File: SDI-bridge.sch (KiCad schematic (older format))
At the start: 95 parts, among them J1 543630489, J2 031-70526-21, J3 3220-10-0100-00, U1 GS2971A, U2 MAX8902B, Y1 ABM7_27.000MH_D2Y_T

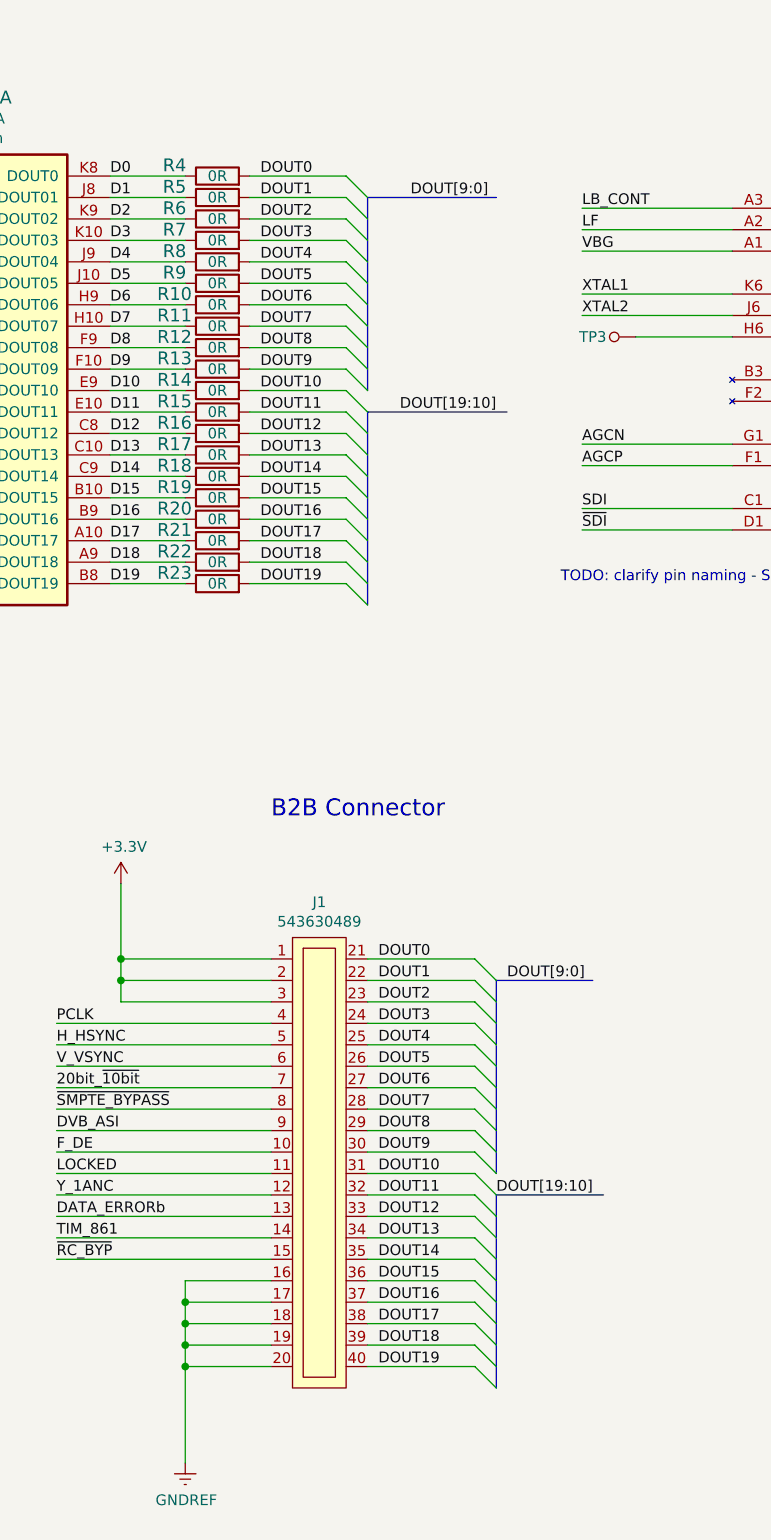
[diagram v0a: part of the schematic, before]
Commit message: Initial routing -WIP
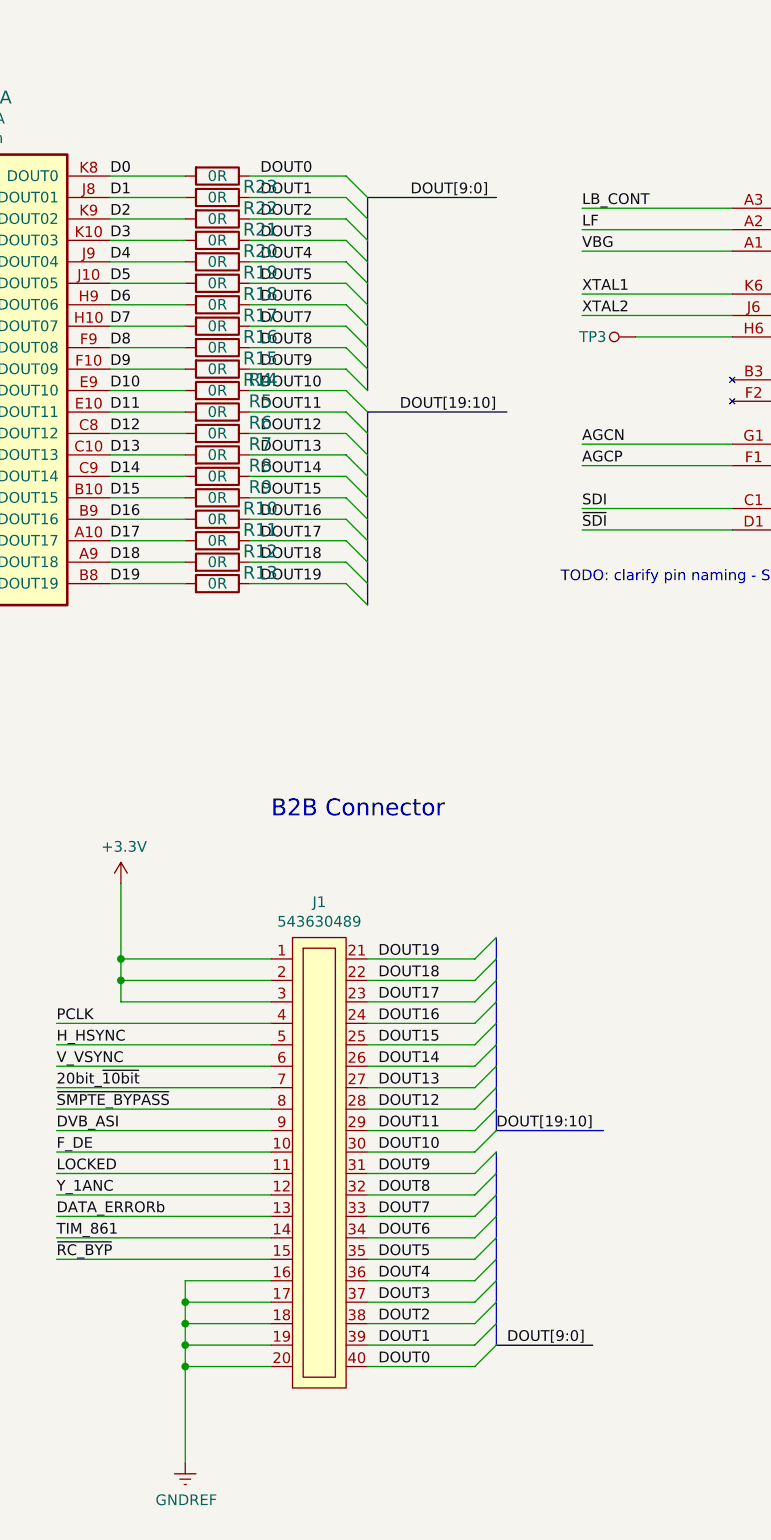
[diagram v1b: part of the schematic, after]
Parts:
- C16: footprint antmicro-footprints:0603 -> antmicro-footprints:0603-cap
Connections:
- net D0: now also R23.2; no longer R4.1
- net D1: now also R22.2; no longer R5.1
- net D10: now also R4.2; no longer R14.1
- net D11: now also R5.2; no longer R15.1
- net D12: now also R6.2; no longer R16.1
- net D13: now also R7.2; no longer R17.1
- net D14: now also R8.2; no longer R18.1
- net D15: now also R9.2; no longer R19.1
- net D16: now also R10.2; no longer R20.1
- net D17: now also R11.2; no longer R21.1
- net D18: now also R12.2; no longer R22.1
- net D19: now also R13.2; no longer R23.1
- net D2: now also R21.2; no longer R6.1
- net D3: now also R20.2; no longer R7.1
- net D4: now also R19.2; no longer R8.1
- net D5: now also R18.2; no longer R9.1
- net D6: now also R17.2; no longer R10.1
- net D7: now also R16.2; no longer R11.1
- net D8: now also R15.2; no longer R12.1
- net D9: now also R14.2; no longer R13.1
- net DOUT0: now also J1.40, R23.1; no longer J1.21, R4.2
- net DOUT1: now also J1.39, R22.1; no longer J1.22, R5.2
- net DOUT10: now also J1.30, R4.1; no longer J1.31, R14.2
- net DOUT11: now also J1.29, R5.1; no longer J1.32, R15.2
- net DOUT12: now also J1.28, R6.1; no longer J1.33, R16.2
- net DOUT13: now also J1.27, R7.1; no longer J1.34, R17.2
- net DOUT14: now also J1.26, R8.1; no longer J1.35, R18.2
- net DOUT15: now also J1.25, R9.1; no longer J1.36, R19.2
- net DOUT16: now also J1.24, R10.1; no longer J1.37, R20.2
- net DOUT17: now also J1.23, R11.1; no longer J1.38, R21.2
- net DOUT18: now also J1.22, R12.1; no longer J1.39, R22.2
- net DOUT19: now also J1.21, R13.1; no longer J1.40, R23.2
- net DOUT2: now also J1.38, R21.1; no longer J1.23, R6.2
- net DOUT3: now also J1.37, R20.1; no longer J1.24, R7.2
- net DOUT4: now also J1.36, R19.1; no longer J1.25, R8.2
- net DOUT5: now also J1.35, R18.1; no longer J1.26, R9.2
- net DOUT6: now also J1.34, R17.1; no longer J1.27, R10.2
- net DOUT7: now also J1.33, R16.1; no longer J1.28, R11.2
- net DOUT8: now also J1.32, R15.1; no longer J1.29, R12.2
- net DOUT9: now also J1.31, R14.1; no longer J1.30, R13.2
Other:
- moved on the sheet: R10, R11, R12, R13, R14, R15, R16, R17, R18, R19, R20, R21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
